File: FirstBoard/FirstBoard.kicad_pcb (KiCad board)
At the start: 2 copper layers, 84.1 x 119.9 mm, 21 parts, among them J0 Battery, J1 MPU0, J10 MPU9, J11 MPU10, J12 MPU11, J13 MPU12, J15 SD_CARD, J2 MPU1, J3 MPU2, J4 MPU3, J5 MPU4, J6 MPU5, J7 MPU6, J8 MPU7, J9 MPU8, U1 ESP32-DEVKIT1-V1-JOAO, U2 LM2596-Board

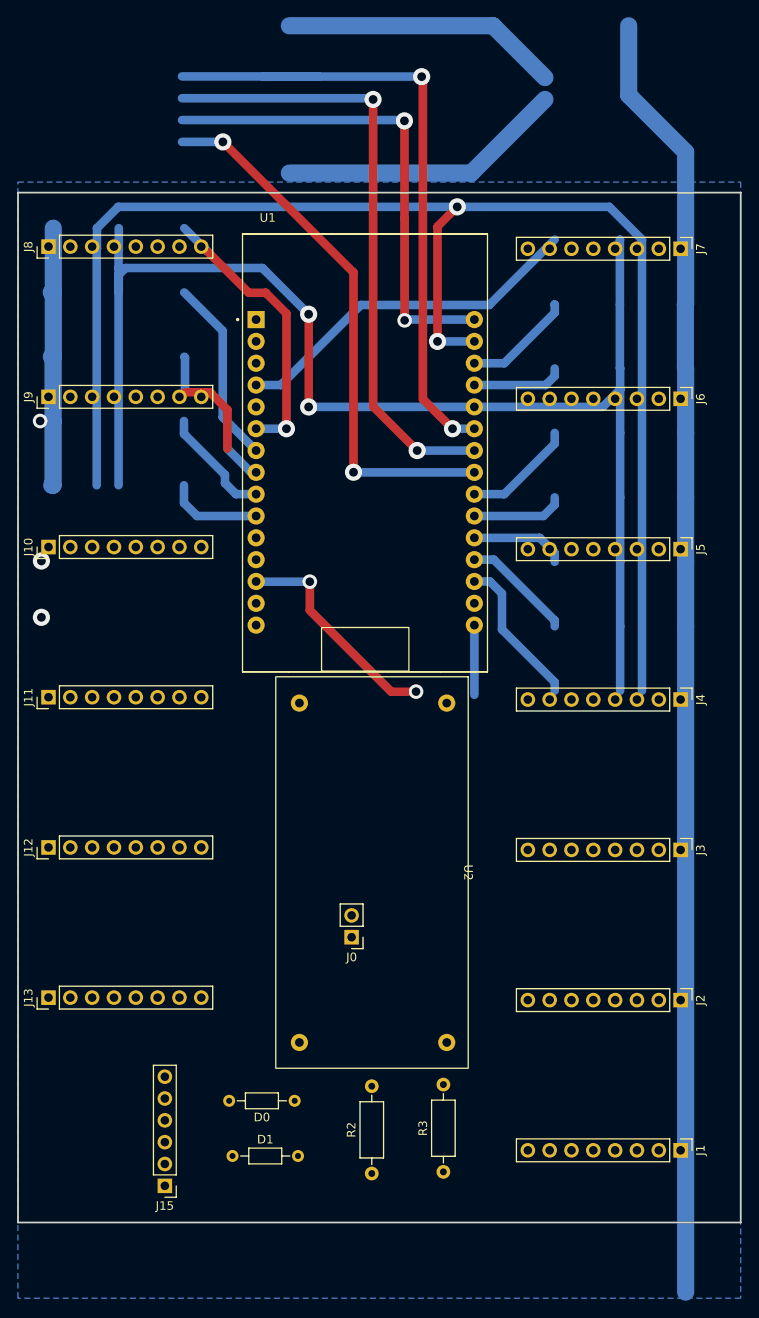
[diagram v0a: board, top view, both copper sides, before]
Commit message: Finished V2
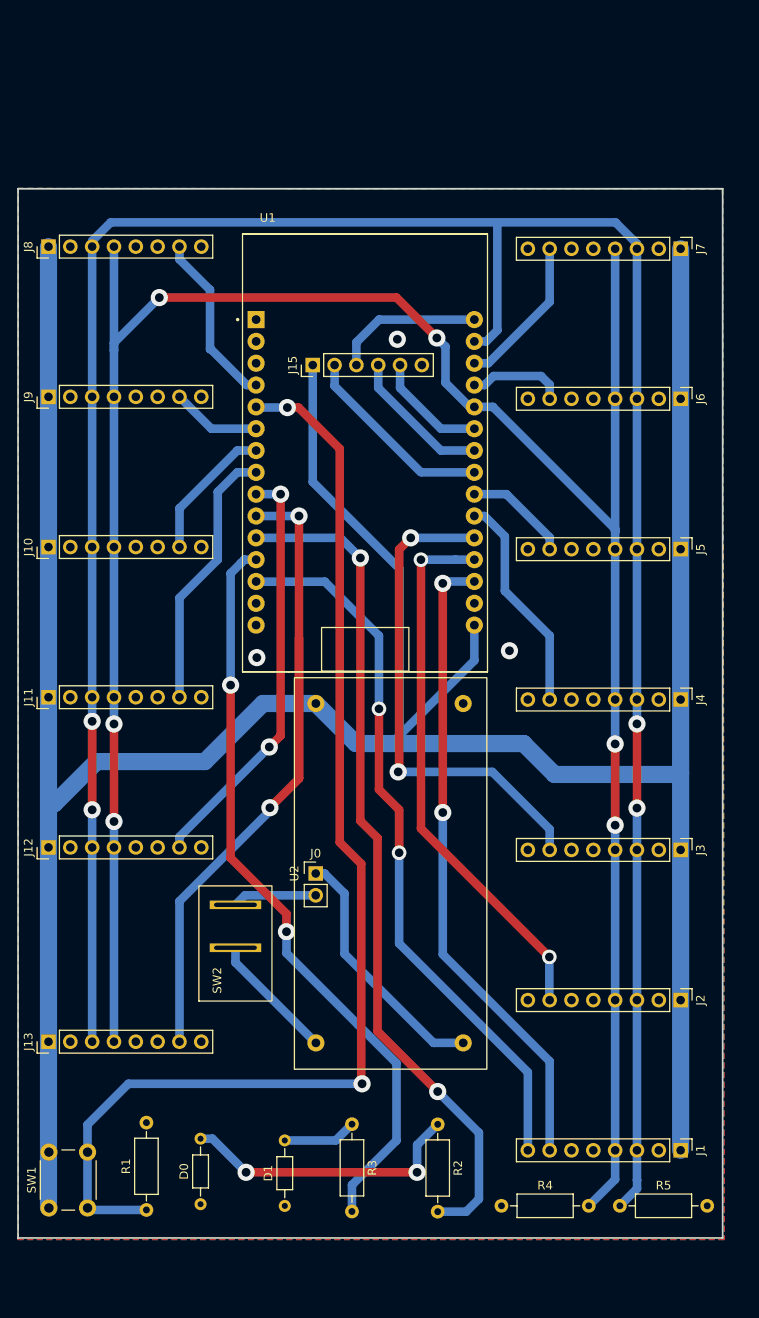
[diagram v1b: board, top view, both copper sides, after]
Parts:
- added R1: 10k, Resistor_THT:R_Axial_DIN0207_L6.3mm_D2.5mm_P10.16mm_Horizontal, F.Cu at (56.1, 179.2)
- added R4: 1K8, Resistor_THT:R_Axial_DIN0207_L6.3mm_D2.5mm_P10.16mm_Horizontal, F.Cu at (97.4, 178.8)
- added R5: 1K8, Resistor_THT:R_Axial_DIN0207_L6.3mm_D2.5mm_P10.16mm_Horizontal, F.Cu at (111.2, 178.8)
- added SW1: SW_Push, Button_Switch_THT:SW_PUSH_6mm_H5mm, F.Cu at (44.8, 179.0)
- added SW2: ON/OFF, TCC_FOOTPRINTS:BOTAO-ONOFF, F.Cu at (66.5, 148.2)
- J3: value MPU2 -> MPU3
- moved J15 97.1 mm to (75.5, 80.9), turned to 90 degrees
- moved D0 16.3 mm to (62.4, 178.6), turned to 90 degrees
- moved R3 12.0 mm to (80.0, 169.3), turned to -90 degrees
- moved R2 9.57 mm to (90.0, 169.3), turned to -90 degrees
- moved J0 8.51 mm to (75.8, 140.1), turned to 0 degrees
- moved D1 8.41 mm to (72.2, 178.8), turned to 90 degrees
- moved J13 5.13 mm to (44.7, 159.7)
- moved U2 1.91 mm to (84.4, 140.0), turned to 90 degrees
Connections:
- U1 pad 1: Net-(J14-Pad5) -> unconnected-(U1-Pad1)
- U1 pad 15: Net-(J14-Pad1) -> unconnected-(U1-Pad15)
- U1 pad 2: Net-(J14-Pad4) -> unconnected-(U1-Pad2)
- U1 pad 3: Net-(J14-Pad3) -> unconnected-(U1-Pad3)
- U1 pad 5: Net-(J14-Pad2) -> Switch
- U2 pad 1: BAT+ -> Net-(U2-Pad1)
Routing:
- net 3v3: track 189.0 -> 363.9 mm, vias 2 -> 0
- net Switch: track 0.00 -> 137.3 mm, vias 0 -> 2
- net SDA: track 157.1 -> 280.5 mm, vias 2 -> 6
- net SCL: track 169.4 -> 287.0 mm, vias 2 -> 4
- net LED_R: track 0.00 -> 98.8 mm, vias 0 -> 2
- net LED_G: track 0.00 -> 88.3 mm, vias 0 -> 2
- net AD0_12: track 11.1 -> 88.4 mm, vias 0 -> 2
- net MISO: track 79.4 -> 13.3 mm, vias 2 -> 0
- net INT: track 25.9 -> 84.0 mm
- net AD0_0: track 17.6 -> 74.9 mm, vias 0 -> 2
- net SCK: track 71.9 -> 16.9 mm, vias 2 -> 0
- net AD0_1: track 13.0 -> 63.7 mm, vias 0 -> 2
- net AD0_2: track 11.1 -> 58.1 mm, vias 0 -> 2
- net SS: track 63.6 -> 22.6 mm, vias 2 -> 0
- net MOSI: track 57.3 -> 17.5 mm, vias 2 -> 0
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- added copper zone on F.Cu, net GND
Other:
- board size 84.1 x 119.9 mm -> 82 x 122.1 mm
